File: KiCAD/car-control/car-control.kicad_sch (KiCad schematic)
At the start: 24 parts, among them J1 Conn_02x03_Odd_Even, J2 Conn_01x06, SW1 SW_Push, SW2 COM-15140, SW2 SW_Push, SW3 SW_Push, SW4 SW_Push, U3 ATmega328-P

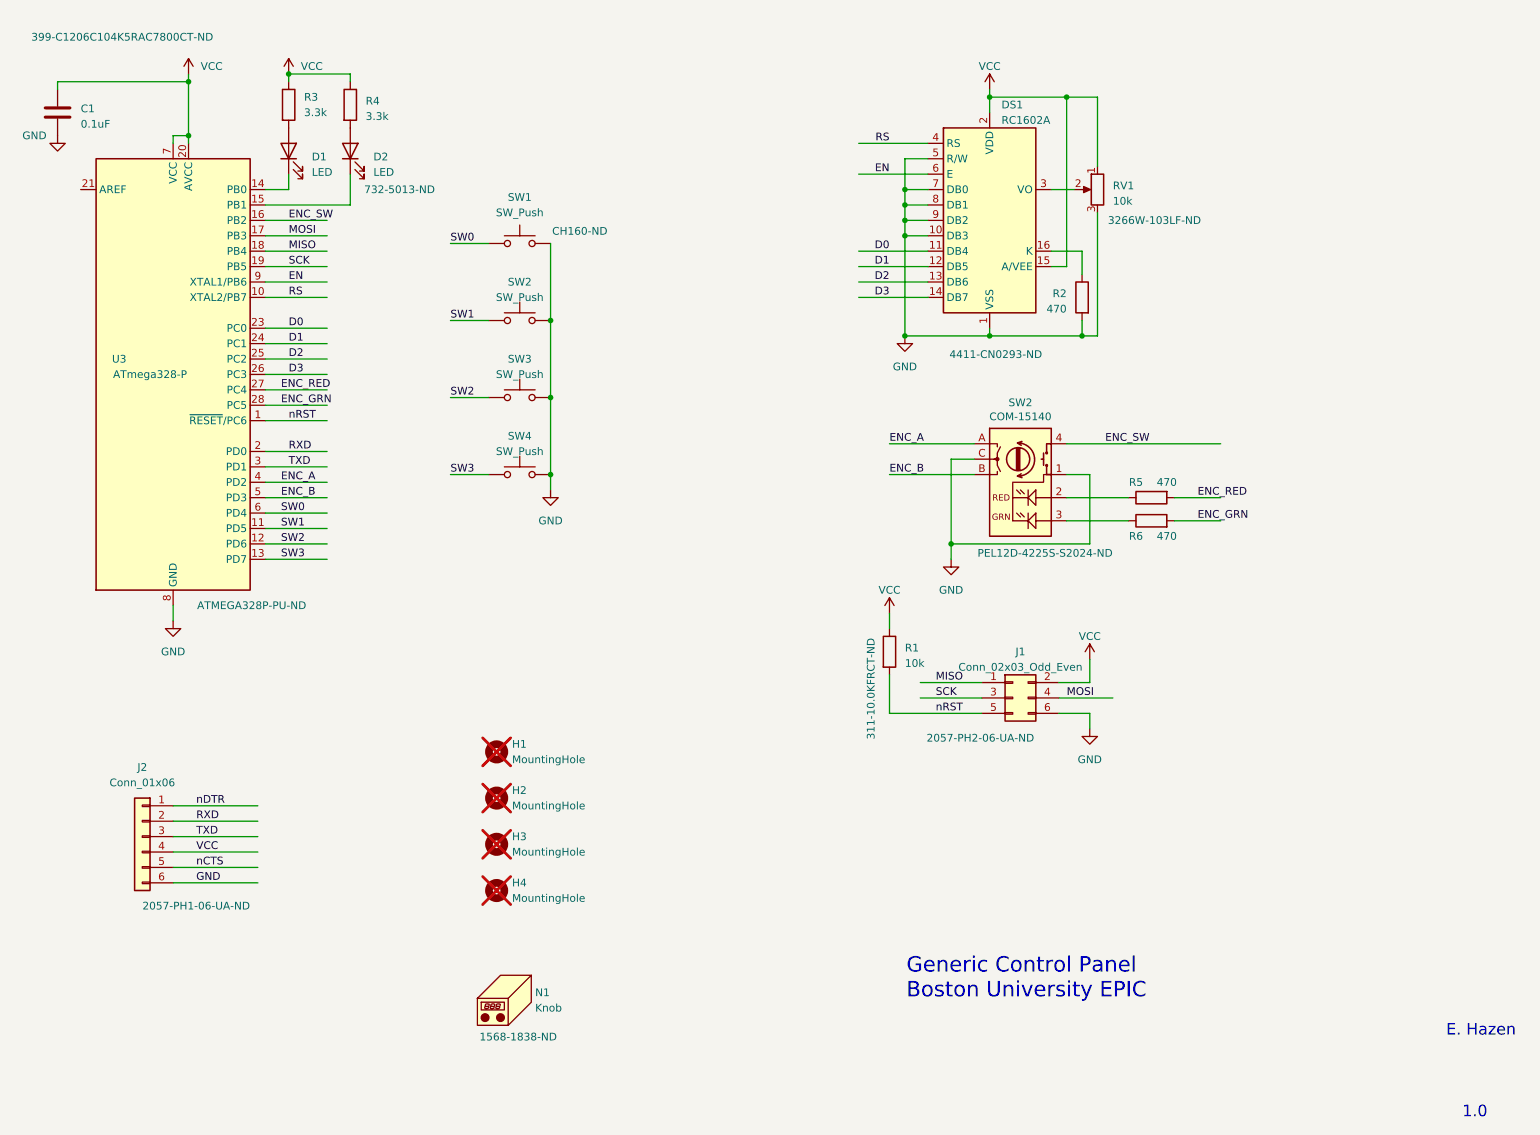
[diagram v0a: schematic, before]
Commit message: working on PCB
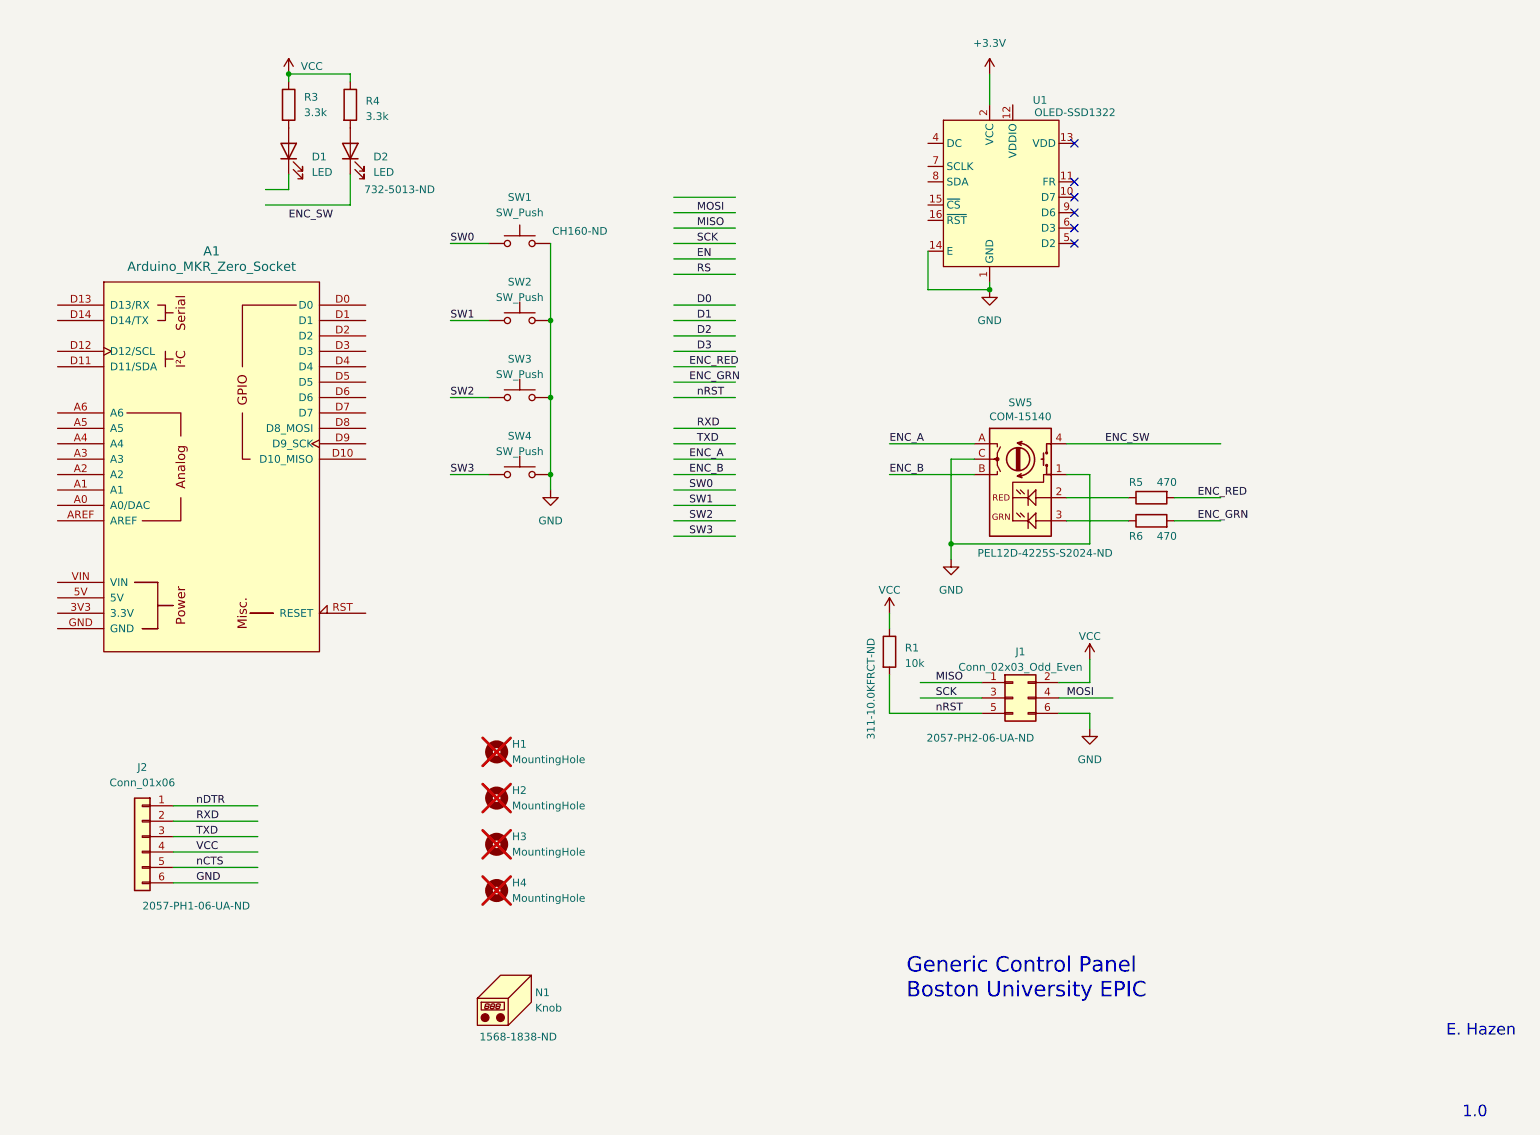
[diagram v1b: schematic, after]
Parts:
- removed C1: 0.1uF, Capacitor_SMD:C_1206_3216Metric_Pad1.33x1.80mm_HandSolder, symbol Device:C
- removed DS1: RC1602A, Display:WC1602A, symbol Display_Character:RC1602A
- removed R2: 470, Resistor_SMD:R_1206_3216Metric_Pad1.30x1.75mm_HandSolder, symbol Device:R
- removed RV1: 10k, Potentiometer_THT:Potentiometer_Bourns_3266W_Vertical, symbol Device:R_Potentiometer
- removed U3: ATmega328-P, Package_DIP:DIP-28_W7.62mm, symbol MCU_Microchip_ATmega:ATmega328-P
- added A1: Arduino_MKR_Zero_Socket, PCM_arduino-library:Arduino_MKR_Zero_Socket, symbol arduino-library:Arduino_MKR_Zero_Socket
- added U1: OLED-SSD1322, symbol my_oled:oled_16p
- renumbered SW2 to SW5
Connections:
- net GND: now also U1.1 (GND), U1.14 (E)
- new net +3.3V: U1.2 (VCC)
- no-connect marks 0 -> 6

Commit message: working on layout
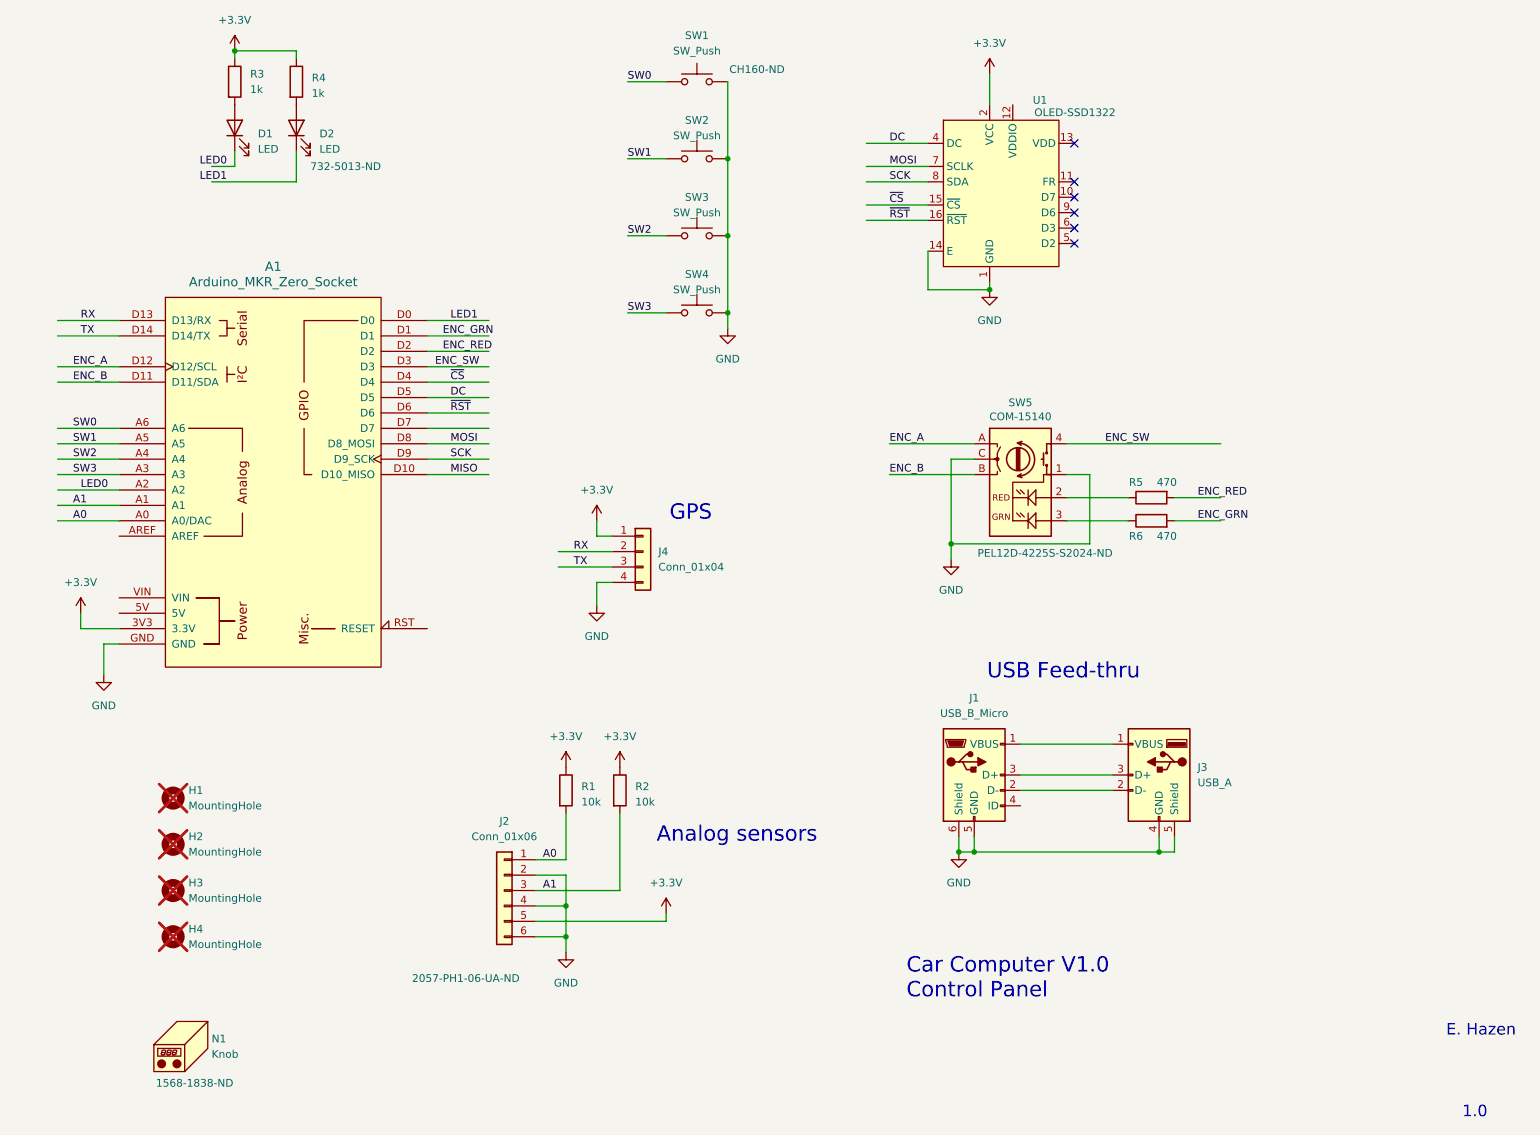
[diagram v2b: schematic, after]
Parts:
- removed J1: Conn_02x03_Odd_Even, Connector_PinHeader_2.54mm:PinHeader_2x03_P2.54mm_Vertical, symbol Connector_Generic:Conn_02x03_Odd_Even
- added J1: USB_B_Micro, my_USB:CONN_USB3131-30-0230-A_GCT, symbol Connector:USB_B_Micro
- added J3: USB_A, my_USB:CONN_USB-A-S-VT_ADM, symbol Connector:USB_A
- added J4: Conn_01x04, Connector_PinSocket_2.54mm:PinSocket_1x04_P2.54mm_Vertical, symbol Connector_Generic:Conn_01x04
- added R2: 10k, Resistor_SMD:R_1206_3216Metric_Pad1.30x1.75mm_HandSolder, symbol Device:R
- R1: CatNo 311-10.0KFRCT-ND -> (none); MfgNo RC1206FR-0710KL -> (none)
- R3, R4: value 3.3k -> 1k
- U1: footprint (none) -> my_OLED:OLED_312_16pin
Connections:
- net RXD is gone; now on net GND: J2.2 (Pin_2)
- net TXD is gone; now on net A1: J2.3 (Pin_3)
- net nCTS is gone; now on net +3.3V: J2.5 (Pin_5)
- net nDTR is gone; now on net A0: J2.1 (Pin_1)
- net nRST is gone; now on net A0: R1.2
- net +3.3V: now also A1.3V3 (3.3V), R1.1, R3.1, R4.1, J4.1 (Pin_1), R2.1
- net ENC_A: now also A1.D12 (D12/SCL)
- net ENC_B: now also A1.D11 (D11/SDA)
- net ENC_GRN: now also A1.D1
- net ENC_RED: now also A1.D2
- net ENC_SW: now also A1.D3
- net GND: now also A1.GND, J2.4 (Pin_4), J1.5 (GND), J1.6 (Shield), J3.4 (GND), J3.5 (Shield), J4.4 (Pin_4)
- net MISO: now also A1.D10 (D10_MISO)
- net MOSI: now also A1.D8 (D8_MOSI), U1.7 (SCLK)
- net SCK: now also A1.D9 (D9_SCK), U1.8 (SDA)
- net SW0: now also A1.A6
- net SW1: now also A1.A5
- net SW2: now also A1.A4
- net SW3: now also A1.A3
- net LED1: now reaches D2.1 (K)
- net LED1: now also A1.D0
- net LED0: now reaches D1.1 (K)
- net LED0: now also A1.A2
- net ~{CS}: now reaches U1.15 (~{CS})
- net ~{CS}: now also A1.D4
- net ~{RST}: now reaches U1.16 (~{RST})
- net ~{RST}: now also A1.D6
- net DC: now reaches U1.4 (DC)
- net DC: now also A1.D5
- net A0: now reaches A1.A0 (A0/DAC)
- net A1: now reaches A1.A1
- net A1: now also R2.2
- net RX: now reaches A1.D13 (D13/RX)
- net RX: now also J4.2 (Pin_2)
- net TX: now reaches A1.D14 (D14/TX)
- net TX: now also J4.3 (Pin_3)
- removed net VCC: J2.4 (Pin_4), R1.1, R3.1, R4.1
- new net: J1.1 (VBUS), J3.1 (VBUS)
- new net: J1.2 (D-), J3.2 (D-)
- new net: J1.3 (D+), J3.3 (D+)
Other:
- note added: "Analog sensors"
- note added: "Car Computer V1.0 Control Panel"
- note added: "GPS"
- note added: "USB Feed-thru"
- note removed: "Generic Control Panel Boston University EPIC"
- moved on the sheet: A1, D1, D2, H1, H2, H3, H4, J2, N1, R3, R4, SW1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
